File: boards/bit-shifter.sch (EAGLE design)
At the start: 6 parts, among them SW1 CT10-XXXX-A2, SW2 CT10-XXXX-A2, SW3 CT10-XXXX-A2

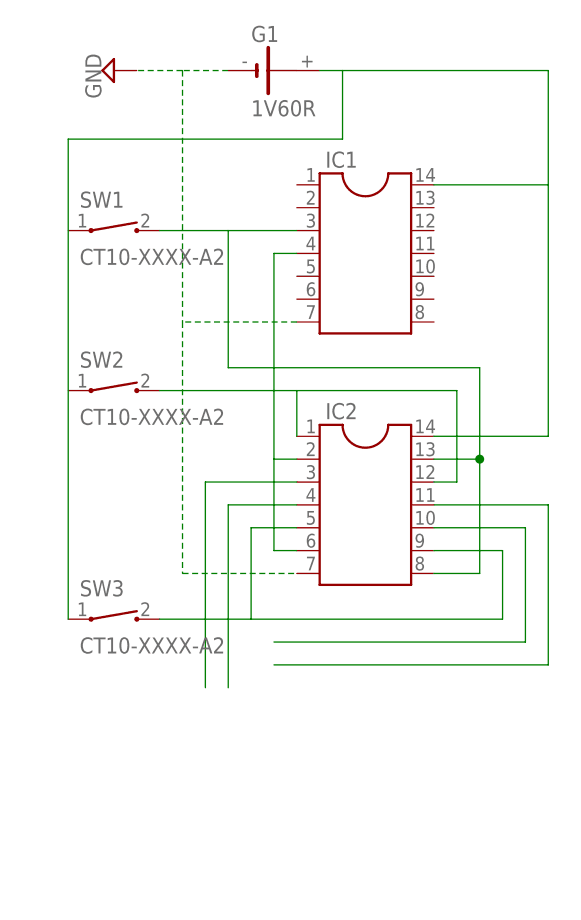
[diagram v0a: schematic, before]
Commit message: Backup before changing timing diagram
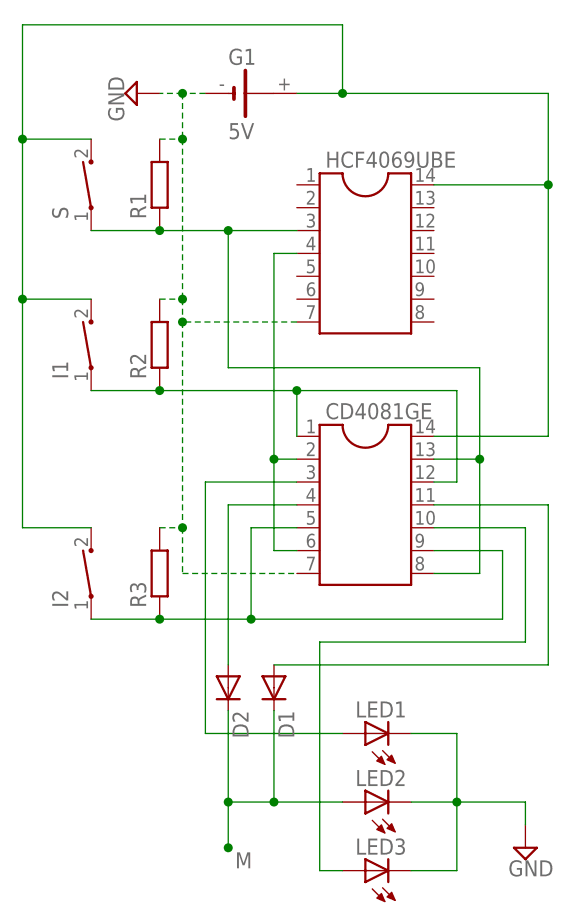
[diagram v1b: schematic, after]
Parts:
- removed SW1, SW2, SW3: CT10-XXXX-A2, switch-coto:CT10-XXXX-A2
- added D1, D2: 1N4446, diode:1N4446
- added I1, I2, S: CT10-XXXX-A2, switch-coto:CT10-XXXX-A2
- added LED1, LED2, LED3: LAP4-BOTTOM, led:LAP4-BOTTOM
- added R1, R2, R3: (no value), resistor:R-EU_0204/2V
- G1: value 1V60R -> 5V
- renumbered IC1 to HCF4069UBE, IC2 to CD4081GE
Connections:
- removed net N$3: CD4081GE.13, CD4081GE.8, HCF4069UBE.3, SW1.2
- removed net N$7: CD4081GE.1, CD4081GE.12, SW2.2
- new net CD4081: CD4081GE.1, CD4081GE.12, I1.1, R2.1
- new net R5: CD4081GE.13, CD4081GE.8, HCF4069UBE.3, R1.1, S.1
- net GND: now also LED1.C, LED2.C, LED3.C, R1.2, R2.2, R3.2
- net N$1: now also CD4081GE.14, G1.+, I1.2, I2.2, S.2
- net N$11: now also D2.A
- net N$2: now also D1.C, D2.C, LED2.A; no longer CD4081GE.14, G1.+, SW3.1
- net N$4: now also I2.1, R3.1; no longer SW3.2
- net N$5: now also LED3.A
- net N$6: now also D1.A
- net N$9: now also LED1.A
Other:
- note added: "M"
- moved on the sheet: G1
